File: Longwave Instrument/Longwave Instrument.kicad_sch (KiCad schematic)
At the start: 45 parts, among them U13 X, U8 ADR510, U9 LM4040B

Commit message: SpectDrone Development
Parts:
- R10, RS2, RS5, R_{PD}1, R_{PD}2, U13: now left out of the parts list
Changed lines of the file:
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@@
   )
   (symbol (lib_id "Device:R") (at 114.3 53.975 0) (unit 1)
-    (in_bom yes) (on_board yes)
+    (in_bom no) (on_board yes)
     (property "Reference" "RS2" (id 0) (at 115.57 52.705 0)
       (effects (font (size 1.27 1.27)) (justify left))
@@
   )
   (symbol (lib_id "Device:R") (at 96.52 84.455 0) (unit 1)
-    (in_bom yes) (on_board yes)
+    (in_bom no) (on_board yes)
     (property "Reference" "R_{PD}2" (id 0) (at 90.805 81.28 0)
       (effects (font (size 1.27 1.27)) (justify left))
@@
   )
   (symbol (lib_id "Device:R") (at 96.52 53.975 0) (unit 1)
-    (in_bom yes) (on_board yes)
+    (in_bom no) (on_board yes)
     (property "Reference" "R_{PD}1" (id 0) (at 90.805 50.8 0)
       (effects (font (size 1.27 1.27)) (justify left))
@@
   )
   (symbol (lib_id "Device:R") (at 114.3 84.455 0) (unit 1)
-    (in_bom yes) (on_board yes)
+    (in_bom no) (on_board yes)
     (property "Reference" "RS5" (id 0) (at 115.57 83.185 0)
       (effects (font (size 1.27 1.27)) (justify left))
@@
   )
   (symbol (lib_id "Device:R") (at 230.505 82.55 270) (mirror x) (unit 1)
-    (in_bom yes) (on_board yes)
+    (in_bom no) (on_board yes)
     (property "Reference" "R10" (id 0) (at 230.505 80.01 90))
     (property "Value" "X" (id 1) (at 230.505 82.55 90))
@@
   )
   (symbol (lib_id "Gardenuino_Custom:ADR510") (at 238.125 86.995 270) (mirror x) (unit 1)
-    (in_bom yes) (on_board yes)
+    (in_bom no) (on_board yes)
     (property "Reference" "U13" (id 0) (at 236.22 85.725 90)
       (effects (font (size 1.27 1.27)) (justify right))

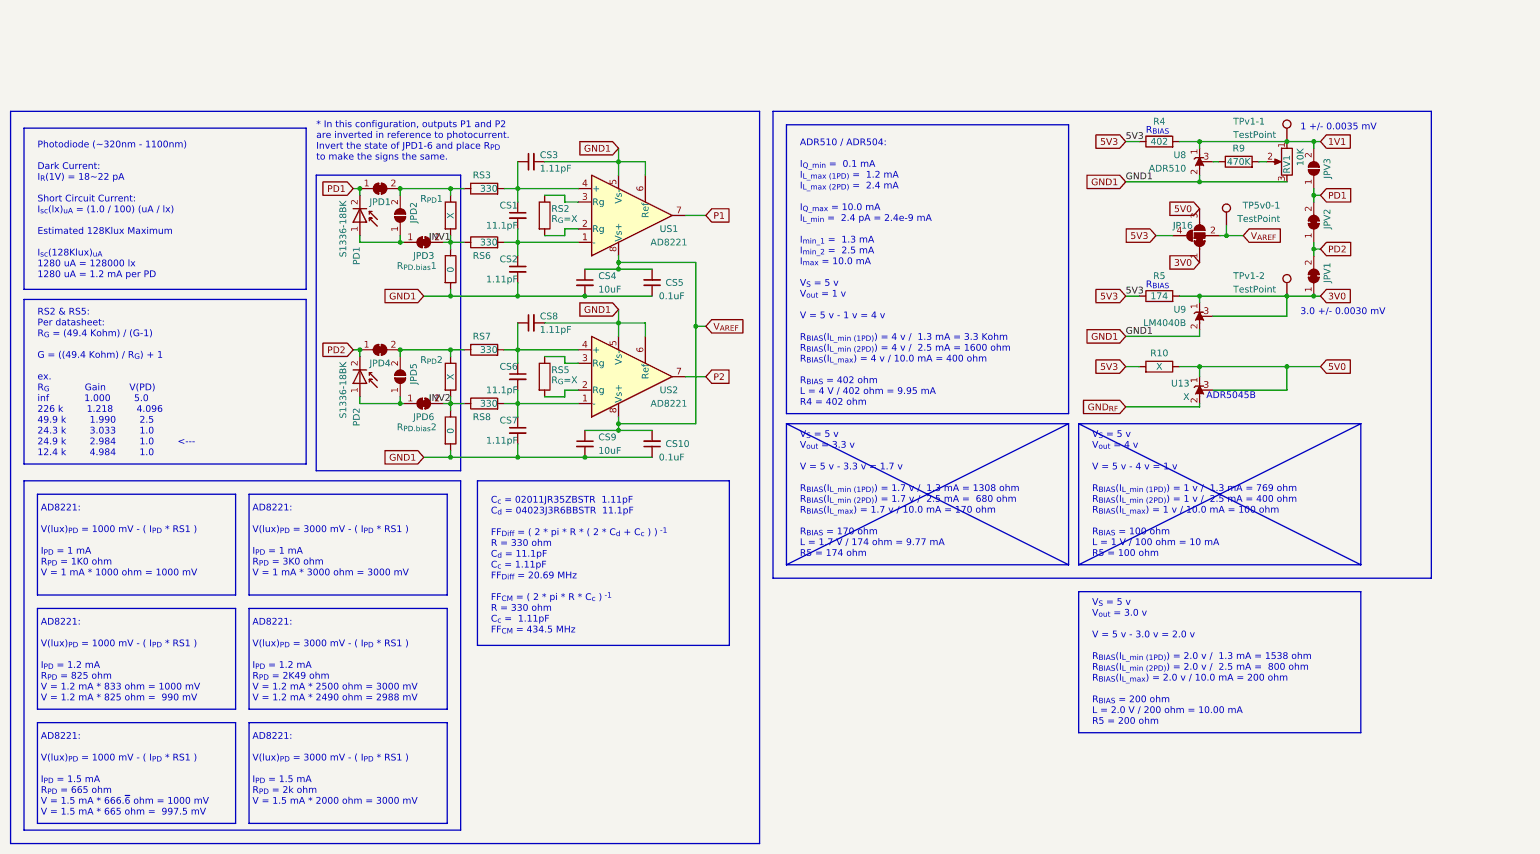
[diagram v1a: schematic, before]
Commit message: SpectDrone Development
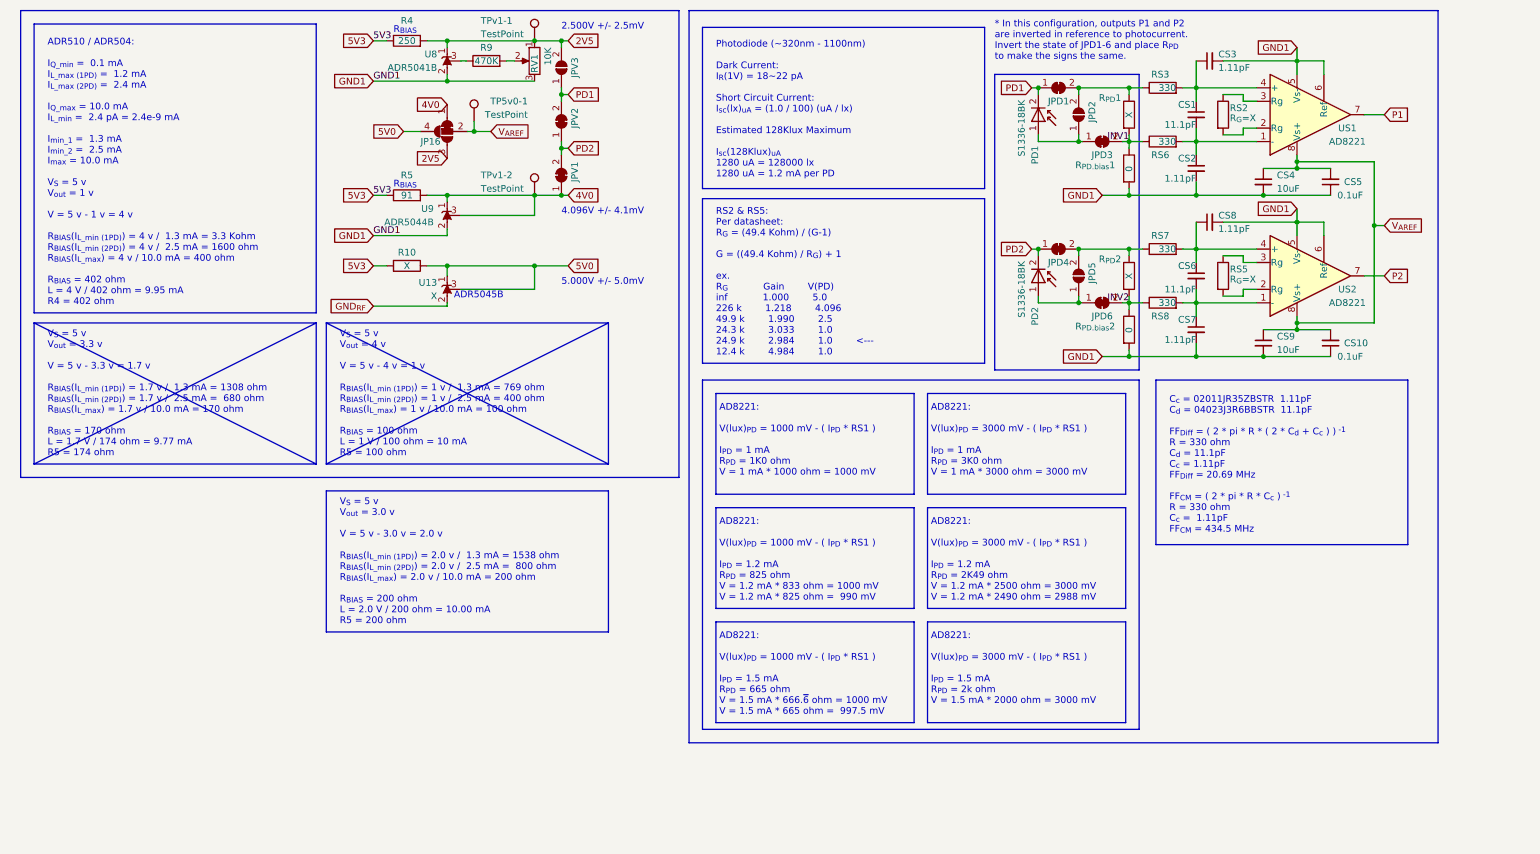
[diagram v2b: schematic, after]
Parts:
- R4: value 402 -> 250; Part Number ERJ-6ENF4020V -> ERJ-PB6B2490V
- R5: value 174 -> 91; Part Number ERJ-6ENF1740V -> CRCW080591R0FKEAHP
- U8: value ADR510 -> ADR5041B
- U9: value LM4040B -> ADR5044B
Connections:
- net 5V0: now also JP16.4 (B); no longer JP16.3 (B)
- net 5V3: no longer JP16.4 (B)
- net 1V1 renamed 2V5
- net 2V5: now also JP16.3 (B)
- net 3V0 renamed 4V0
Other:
- note added: "2.500V +/- 2.5mV"
- note added: "4.096V +/- 4.1mV"
- note added: "5.000V +/- 5.0mV"
- note removed: "1 +/- 0.0035 mV"
- note removed: "3.0 +/- 0.0030 mV"
- moved on the sheet: CS1, CS10, CS2, CS3, CS4, CS5, CS6, CS7, CS8, CS9, JP16, JPD1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
